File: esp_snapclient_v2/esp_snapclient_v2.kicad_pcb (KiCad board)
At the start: 2 copper layers, 30 parts, among them J1 USB_C_Receptacle_PowerOnly_6P, J2 Screw_Terminal_01x04, J3 Conn_01x04_Socket, SW1 SW_Push, SW2 SW_Push, U1 ESP32-WROVER-E, U2 MAX98357A, U3 MAX98357A, U5 AMS1117-3.3

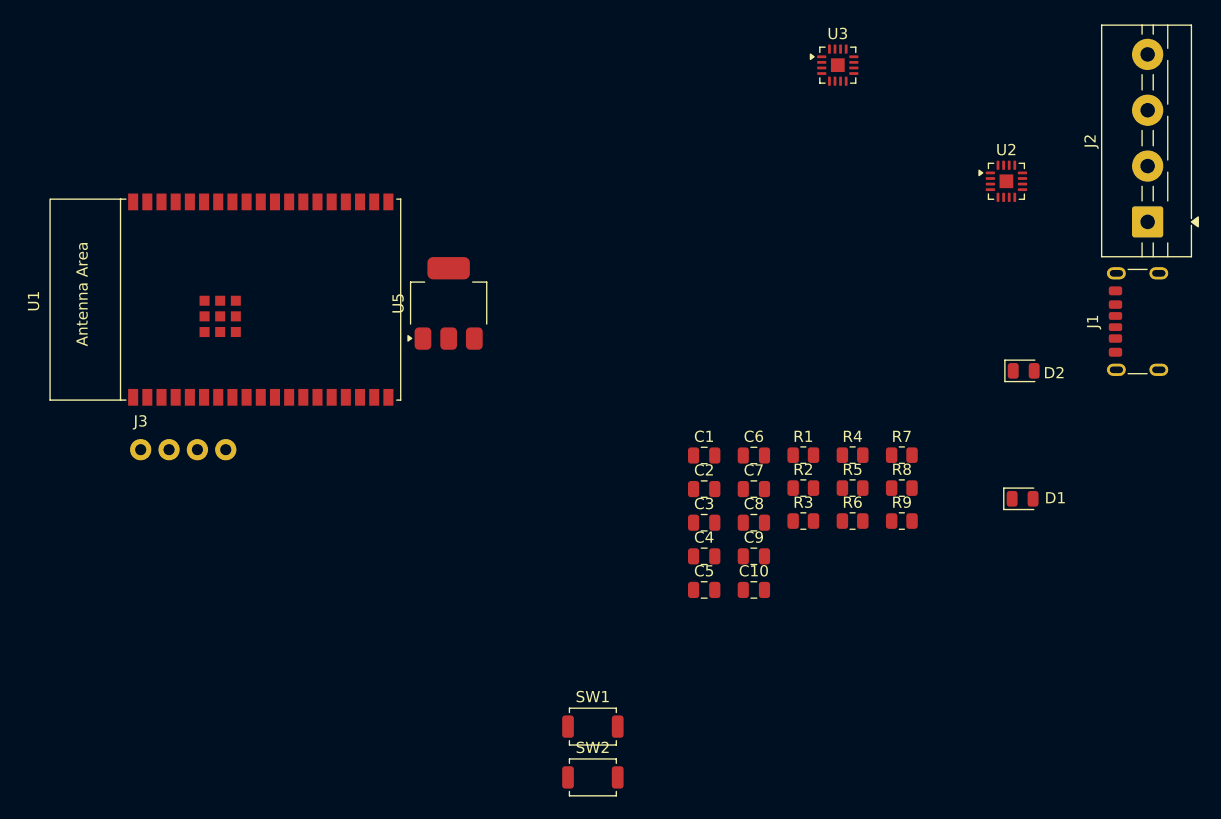
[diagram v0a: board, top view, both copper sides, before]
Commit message: feat: up
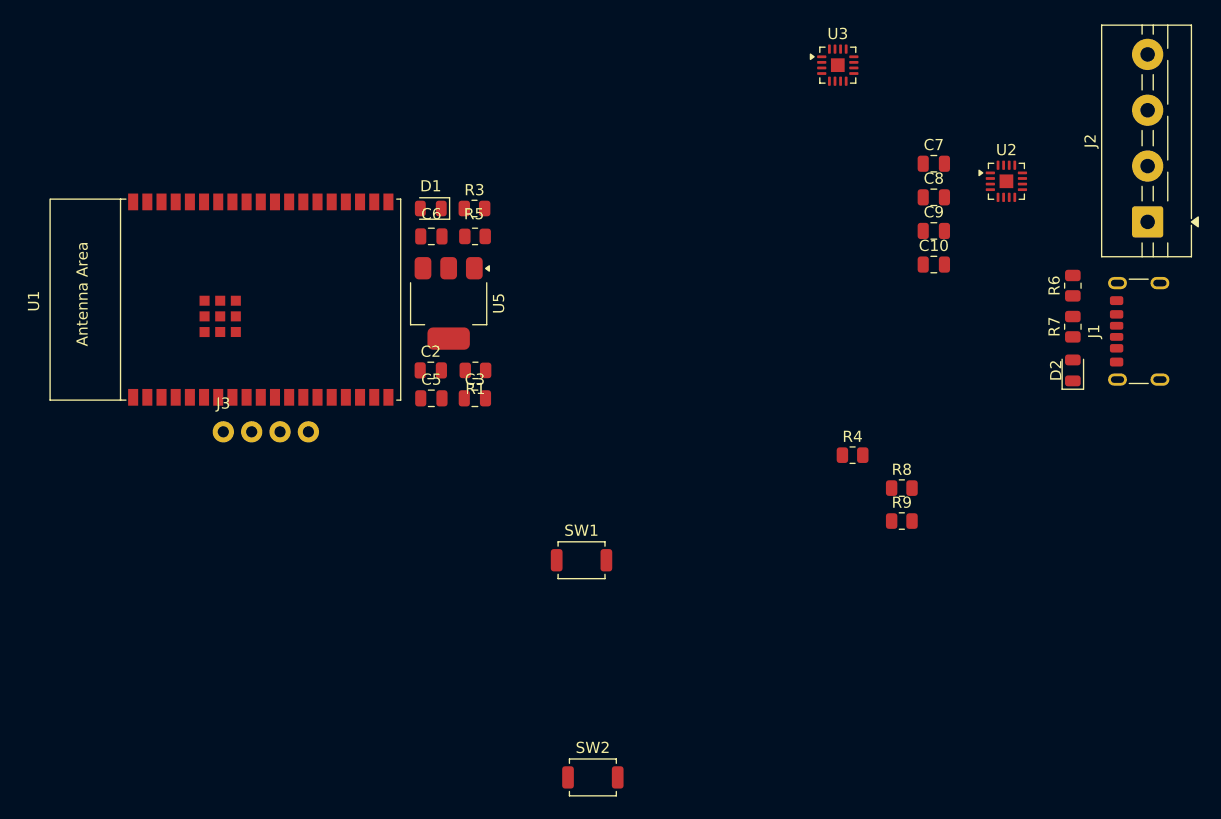
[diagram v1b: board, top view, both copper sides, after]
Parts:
- removed C1: 22uF, Capacitor_SMD:C_0805_2012Metric
- removed C4: 0.1uF, Capacitor_SMD:C_0805_2012Metric
- removed R2: 0R, Resistor_SMD:R_0805_2012Metric
- moved D1 59.0 mm to (103.5, 49.0), turned to 180 degrees
- moved R5 40.6 mm to (107.5, 51.5), turned to 180 degrees
- moved R3 40.6 mm to (107.4, 49.0)
- moved C6 34.9 mm to (103.5, 51.5)
- moved C9 33.3 mm to (148.6, 51.0)
- moved C10 33.3 mm to (148.6, 54.0)
- moved C7 33.3 mm to (148.6, 45.0)
- moved C8 33.3 mm to (148.6, 48.0)
- moved R1 30.3 mm to (107.5, 63.5), turned to 180 degrees
- moved C5 29.9 mm to (103.5, 66.0)
- moved R6 28.9 mm to (161.0, 55.9), turned to 90 degrees
- moved C2 26.7 mm to (103.5, 63.5)
- moved C3 23.4 mm to (107.5, 66.0)
- moved R7 19.2 mm to (161.0, 59.6), turned to 90 degrees
- moved SW1 14.9 mm to (117.0, 80.5)
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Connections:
- SW1 pad 1: GND -> /EN
- SW1 pad 2: Net-(C4-Pad2) -> GND
